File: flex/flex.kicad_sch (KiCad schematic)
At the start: 131 parts, among them J1 NA_Conn_01x06_Female, J2 NA_Conn_01x05_Female, J3 NA_Conn_01x06_Female, J4 NA_Conn_01x03_Female, J5 NA_Conn_01x03_Female, SW1 SW_Push, SW10 SW_Push, SW11 SW_Push, SW12 SW_Push, SW13 SW_Push, SW14 SW_Push, SW15 SW_Push, SW16 SW_Push, SW17 SW_Push, SW18 SW_Push, SW19 SW_Push, SW2 SW_Push, SW20 SW_Push, SW21 SW_Push, SW22 SW_Push, SW23 SW_Push, SW24 SW_Push, SW3 SW_Push, SW4 SW_Push, SW5 SW_Push, SW6 SW_Push, SW7 SW_Push, SW8 SW_Push, SW9 SW_Push

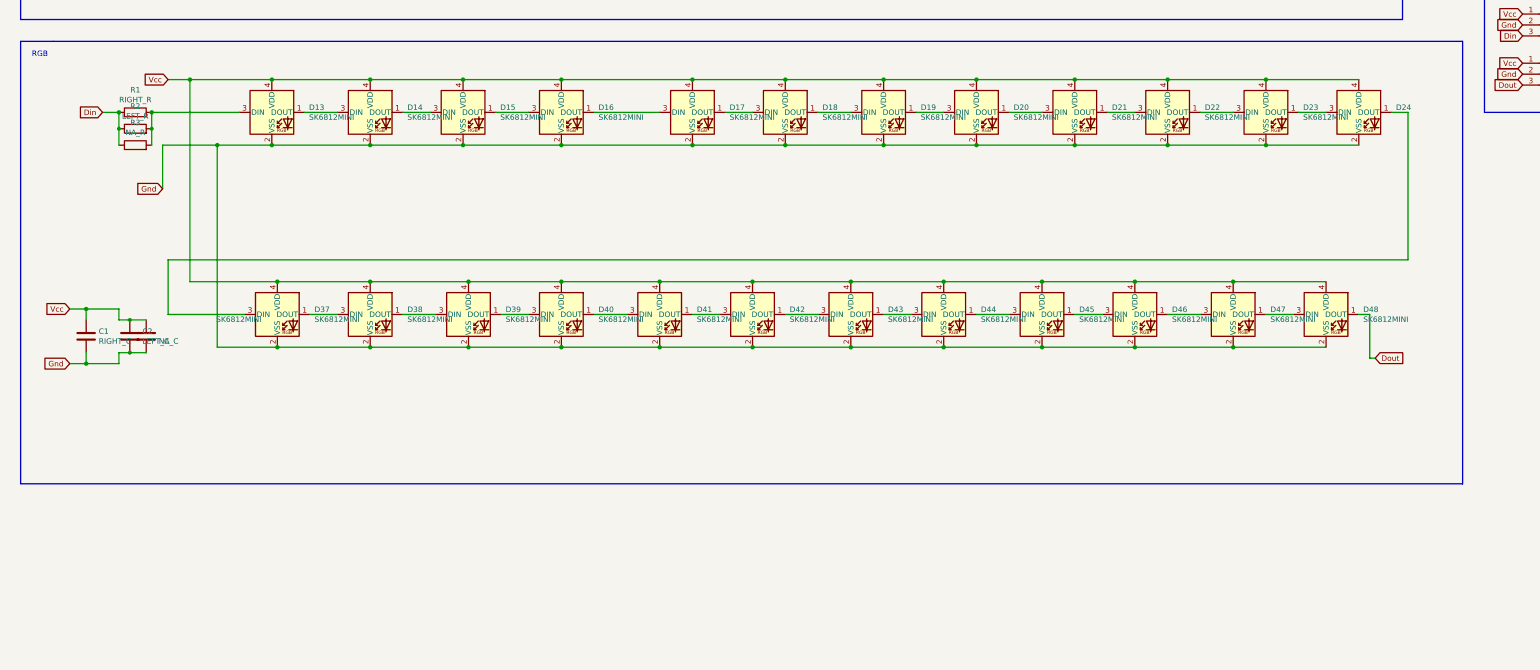
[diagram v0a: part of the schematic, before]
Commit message: LEDs
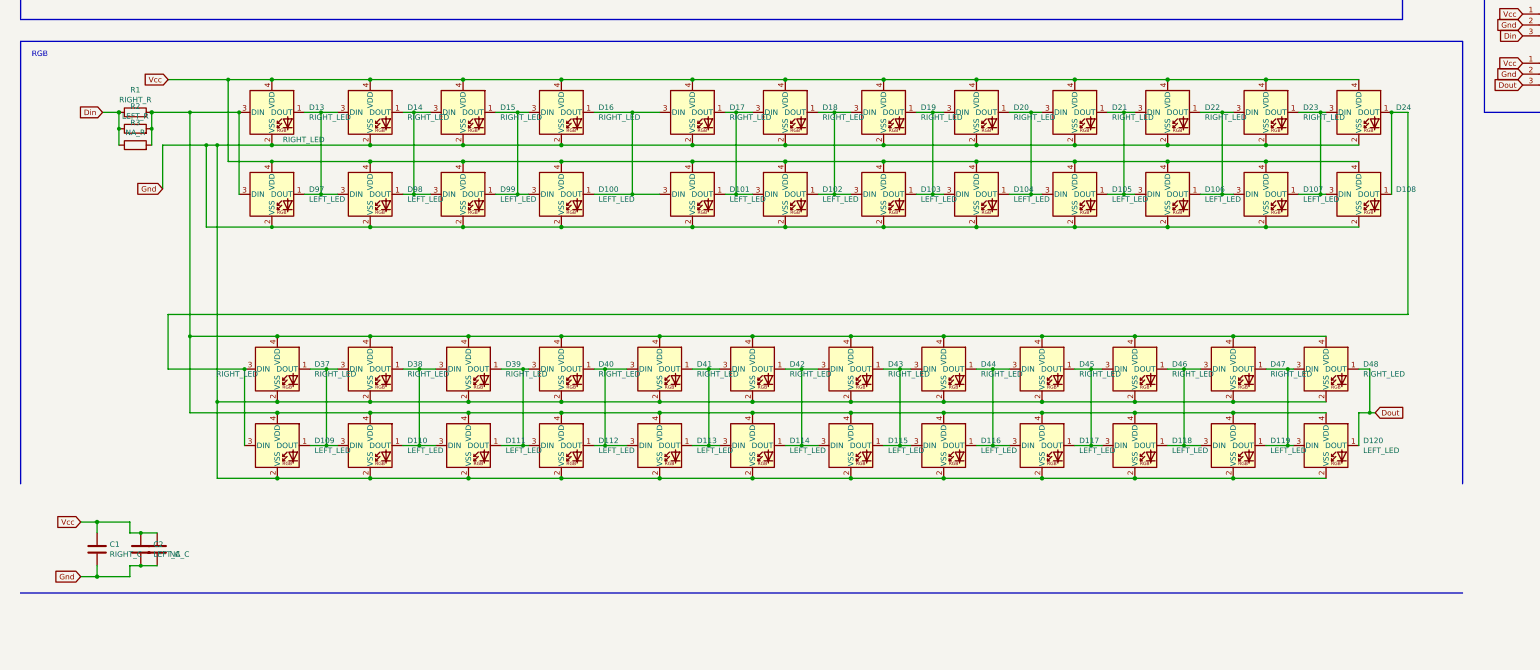
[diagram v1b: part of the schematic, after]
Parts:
- added D100, D101, D102, D103, D104, D105, D106, D107, D109, D110, D111, D112, D113, D114, D115, D116, D117, D118, D119, D120, D97, D98, D99: LEFT_LED, libs:SK6812_mini_e_corners_noedgecuts, symbol LED:SK6812MINI
- added D108: RIGHT_LED, libs:SK6812_mini_e_corners_noedgecuts, symbol LED:SK6812MINI
- D13, D14, D15, D16, D17, D18, D19, D20, D21, D22, D23, D24, D37, D38, D39, D40, D41, D42, D43, D44, D45, D46, D47, D48: value SK6812MINI -> RIGHT_LED
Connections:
- net Dout: now also D120.1 (DOUT)
- net Gnd: now also D100.2 (VSS), D101.2 (VSS), D102.2 (VSS), D103.2 (VSS), D104.2 (VSS), D105.2 (VSS), D106.2 (VSS), D107.2 (VSS), D108.2 (VSS), D109.2 (VSS), D110.2 (VSS), D111.2 (VSS), D112.2 (VSS), D113.2 (VSS), D114.2 (VSS), D115.2 (VSS), D116.2 (VSS), D117.2 (VSS), D118.2 (VSS), D119.2 (VSS), D120.2 (VSS), D97.2 (VSS), D98.2 (VSS), D99.2 (VSS)
- net Vcc: now also D100.4 (VDD), D101.4 (VDD), D102.4 (VDD), D103.4 (VDD), D104.4 (VDD), D105.4 (VDD), D106.4 (VDD), D107.4 (VDD), D108.4 (VDD), D97.4 (VDD), D98.4 (VDD), D99.4 (VDD); no longer D37.4 (VDD), D38.4 (VDD), D39.4 (VDD), D40.4 (VDD), D41.4 (VDD), D42.4 (VDD), D43.4 (VDD), D44.4 (VDD), D45.4 (VDD), D46.4 (VDD), D47.4 (VDD), D48.4 (VDD)
- net at D13.3 (DIN), R1.2, R2.2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: now also D37.4 (VDD), D38.4 (VDD), D39.4 (VDD), D40.4 (VDD), D41.4 (VDD), D42.4 (VDD), D43.4 (VDD), D44.4 (VDD), D45.4 (VDD), D46.4 (VDD), D47.4 (VDD), D48.4 (VDD), D109.4 (VDD), D110.4 (VDD), D111.4 (VDD), D112.4 (VDD), D113.4 (VDD), D114.4 (VDD), D115.4 (VDD), D116.4 (VDD), D117.4 (VDD), D118.4 (VDD), D119.4 (VDD), D120.4 (VDD), D97.3 (DIN)
- net at D21.1 (DOUT), D22.3 (DIN): now also D105.1 (DOUT), D106.3 (DIN)
- net at D20.1 (DOUT), D21.3 (DIN): now also D104.1 (DOUT), D105.3 (DIN)
- net at D40.1 (DOUT), D41.3 (DIN): now also D112.1 (DOUT), D113.3 (DIN)
- net at D39.1 (DOUT), D40.3 (DIN): now also D111.1 (DOUT), D112.3 (DIN)
- net at D13.1 (DOUT), D14.3 (DIN): now also D97.1 (DOUT), D98.3 (DIN)
- net at D23.1 (DOUT), D24.3 (DIN): now also D107.1 (DOUT), D108.3 (DIN)
- net at D22.1 (DOUT), D23.3 (DIN): now also D106.1 (DOUT), D107.3 (DIN)
- net at D19.1 (DOUT), D20.3 (DIN): now also D103.1 (DOUT), D104.3 (DIN)
- net at D18.1 (DOUT), D19.3 (DIN): now also D102.1 (DOUT), D103.3 (DIN)
- net at D37.1 (DOUT), D38.3 (DIN): now also D109.1 (DOUT), D110.3 (DIN)
- net at D24.1 (DOUT), D37.3 (DIN): now also D108.1 (DOUT), D109.3 (DIN)
- net at D38.1 (DOUT), D39.3 (DIN): now also D110.1 (DOUT), D111.3 (DIN)
- net at D42.1 (DOUT), D43.3 (DIN): now also D114.1 (DOUT), D115.3 (DIN)
- net at D41.1 (DOUT), D42.3 (DIN): now also D113.1 (DOUT), D114.3 (DIN)
- net at D47.1 (DOUT), D48.3 (DIN): now also D119.1 (DOUT), D120.3 (DIN)
- net at D17.1 (DOUT), D18.3 (DIN): now also D101.1 (DOUT), D102.3 (DIN)
- net at D16.1 (DOUT), D17.3 (DIN): now also D100.1 (DOUT), D101.3 (DIN)
- net at D45.1 (DOUT), D46.3 (DIN): now also D117.1 (DOUT), D118.3 (DIN)
- net at D44.1 (DOUT), D45.3 (DIN): now also D116.1 (DOUT), D117.3 (DIN)
- net at D46.1 (DOUT), D47.3 (DIN): now also D118.1 (DOUT), D119.3 (DIN)
- net at D43.1 (DOUT), D44.3 (DIN): now also D115.1 (DOUT), D116.3 (DIN)
- net at D15.1 (DOUT), D16.3 (DIN): now also D100.3 (DIN), D99.1 (DOUT)
- net at D14.1 (DOUT), D15.3 (DIN): now also D98.1 (DOUT), D99.3 (DIN)
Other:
- moved on the sheet: C1, C2, D37, D38, D39, D40, D41, D42, D43, D44, D45, D46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
